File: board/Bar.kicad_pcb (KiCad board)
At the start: 2 copper layers, 55 x 80 mm, 41 parts, among them J1 SUPPLY, J2 SUPPLY, J3 USB_A, J4 Screw_Terminal_01x02, J5 SUPPLY, J6 SUPPLY, U1 74HC595, U2 74HC595, U3 ATtiny85-20PU

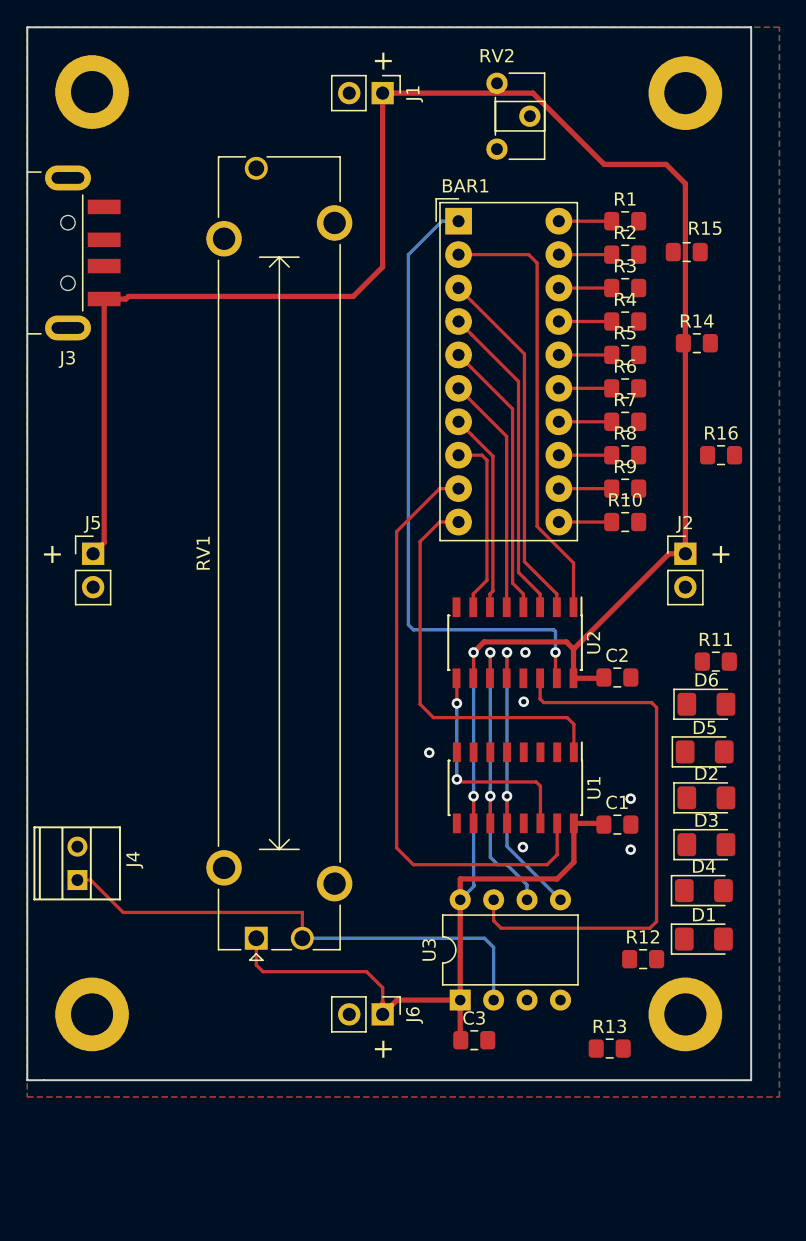
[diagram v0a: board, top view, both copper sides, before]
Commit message: final board
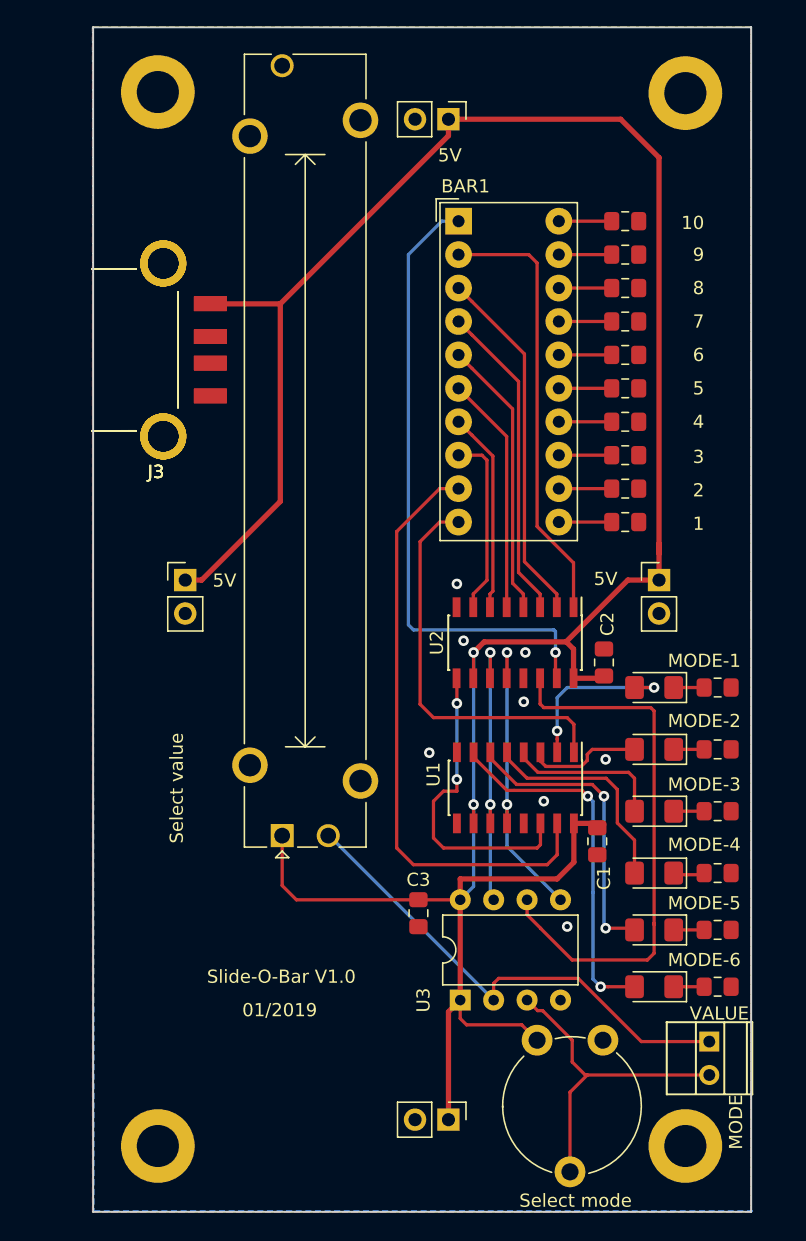
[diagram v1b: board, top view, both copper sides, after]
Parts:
- removed the J3 at (8.26, 29.2)
- added J3 (x3): USB_A, myfootprint:LUM_2410_06_USB_A_SMD, F.Cu at (15.5, 36.6)
- RV2: footprint Potentiometer_THT:Potentiometer_ACP_CA6-H2,5_Horizontal -> Potentiometer_THT:Potentiometer_Piher_PT-10-V10_Vertical
- moved RV2 72.8 mm to (50.8, 89.0), turned to 270 degrees
- moved R15 51.6 mm to (64.5, 80.6)
- moved J4 49.6 mm to (63.9, 89.2), turned to 270 degrees
- moved R16 40.4 mm to (64.5, 85.0)
- moved R14 40.3 mm to (64.5, 76.3)
- moved D6 21.8 mm to (59.7, 85.0), turned to 180 degrees
- moved R13 19.8 mm to (64.5, 71.6)
- moved D1 19.5 mm to (59.7, 62.2), turned to 180 degrees
- moved R12 16.9 mm to (64.5, 66.9)
- moved D5 14.1 mm to (59.7, 80.6), turned to 180 degrees
- moved REF** 11.2 mm to (22.0, 97.1)
- moved C3 10.5 mm to (41.8, 79.4), turned to 270 degrees
- moved REF** 10.0 mm to (61.9, 97.5)
- moved J6 9.43 mm to (44.1, 95.1)
- moved RV1 8.04 mm to (31.4, 73.5)
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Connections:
- J4 pad 2: GND -> /MODE
- U3 pad 6: /CLOCK -> /DATA
- U3 pad 7: /DATA -> /CLOCK
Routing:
- net /OUT_6: track 0.00 -> 27.7 mm, vias 0 -> 2
- net /MODE: track 0.00 -> 25.1 mm
- net /OUT_5: track 0.00 -> 22.6 mm, vias 0 -> 2
- net /OUT_4: track 0.00 -> 16.7 mm
- net /OUT_1: track 0.00 -> 13.3 mm, vias 0 -> 2
- net /OUT_3: track 0.00 -> 12.0 mm
- net /OUT_2: track 0.00 -> 8.79 mm
- net /SHIFT_OUT: track 17.1 -> 23.9 mm
- net +5V: track 205.4 -> 203.0 mm
- net Net-(D5-Pad1): track 0.00 -> 2.31 mm
- net Net-(D6-Pad1): track 0.00 -> 2.31 mm
- net Net-(D4-Pad1): track 0.00 -> 2.31 mm
- net Net-(D3-Pad1): track 0.00 -> 2.31 mm
- net Net-(D2-Pad1): track 0.00 -> 2.31 mm
- net Net-(D1-Pad1): track 0.00 -> 2.31 mm
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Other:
- board size 55 x 80 mm -> 50 x 90 mm
- board text added: "01/2019"
- board text added: "1"
- board text added: "10"
- board text added: "2"
- board text added: "3"
- board text added: "4"
- board text added: "5"
- board text added: "5V"
- board text added: "6"
- board text added: "7"
- board text added: "8"
- board text added: "9"
- board text added: "MODE"
- board text added: "MODE-1"
- board text added: "MODE-2"
- board text added: "MODE-3"
- board text added: "MODE-4"
- board text added: "MODE-5"
- board text added: "MODE-6"
- board text added: "Select mode"
- board text added: "Select value"
- board text added: "Slide-O-Bar V1.0"
- board text added: "VALUE"
- board text removed: "+"
